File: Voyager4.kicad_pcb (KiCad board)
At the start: 2 copper layers, 34.9 x 38.1 mm, 32 parts, among them Q1 Q_NPN_BEC, SW1 SW_Push, U1 ATmega32U2-MU, U2 PRTR5V0U2X, Y1 16MHz

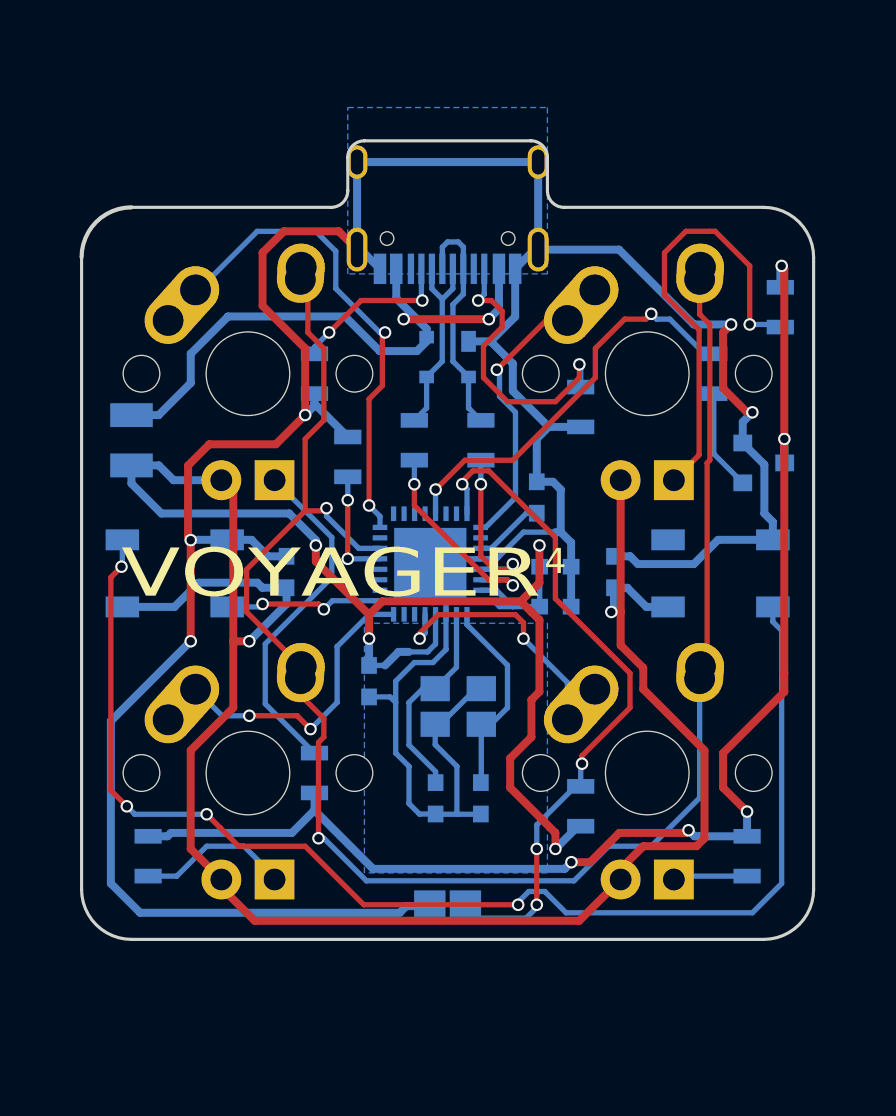
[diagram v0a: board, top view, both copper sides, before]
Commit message: Finish new PCB
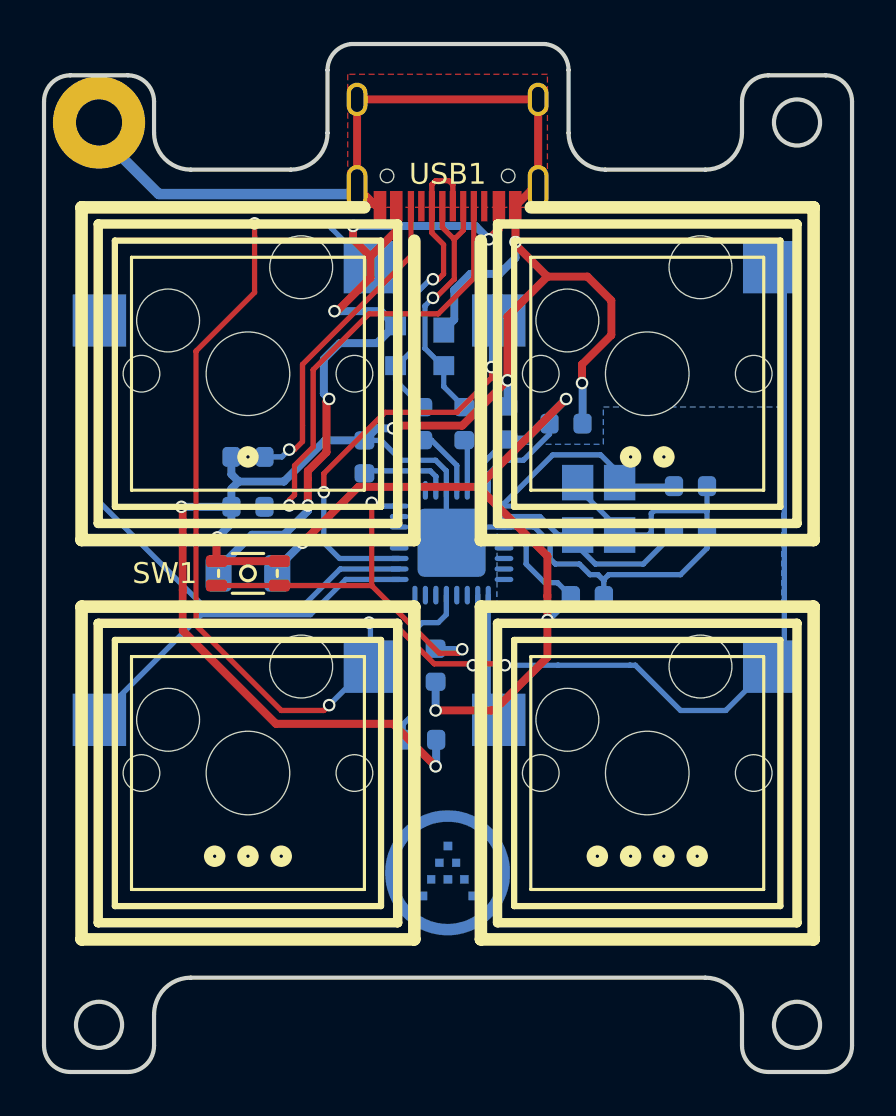
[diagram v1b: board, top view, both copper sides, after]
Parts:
- removed CR1, CR2: 0.1u, Capacitors_SMD:C_0603
- removed D18, D9: WS2812B, LEDs:LED_WS2812B-PLCC4
- removed Q1: Q_NPN_BEC, TO_SOT_Packages_SMD:SOT-23
- removed R10, R27, R7, R8, R9: 1k, Resistors_SMD:R_0805
- added G***: LOGO, locallib:ai-ring-6mm-FancyAss-Mask, B.Cu at (68.3, 63.5)
- added G***: LOGO, locallib:ai-ring-6mm-FancyAss, B.Cu at (68.3, 63.5)
- added GroundingPad: MountingHole_2.2mm_M2_Pad, MountingHole:MountingHole_2.2mm_M2_Pad, F.Cu at (51.6, 27.7)
- added REF**: outline, locallib:outline, F.Cu at (87.8, 25.5)
- C1, C2, C3, C4, C5, C6: footprint Capacitors_SMD:C_0603 -> Capacitor_SMD:C_0603_1608Metric
- F1: footprint Fuse_Holders_and_Fuses:Fuse_SMD1206_Reflow -> Fuse:Fuse_1206_3216Metric
- MX1, MX2, MX3, MX4: footprint MX_Alps_Hybrid:MX-1U -> locallib:MXOnly-1U-Hotswap
- R1, R2, R3, R4, R5, R6: footprint Resistors_SMD:R_0805 -> Resistor_SMD:R_0603_1608Metric
- SW1: footprint random-keyboard-parts:Jumper-UserFriendly-Small -> locallib:Alps-SKSV-LargerPads; moved to F.Cu
- U1: footprint Housings_DFN_QFN:QFN-32-1EP_5x5mm_Pitch0.5mm -> locallib:QFN-32-1EP_5x5mm_Pitch0.5mm
- U2: footprint random-keyboard-parts:SOT143B -> locallib:SOT143B
- USB1: moved to F.Cu
- Y1: footprint Crystals:Crystal_SMD_3225-4pin_3.2x2.5mm -> locallib:Crystal_SMD_3225-4pin_3.2x2.5mm
- moved SW1 18.5 mm to (58.7, 49.2), turned to 0 degrees
- moved C1 17.9 mm to (79.9, 45.1), turned to 0 degrees
- moved C2 17.6 mm to (79.9, 47.2), turned to 0 degrees
- moved R4 16.1 mm to (58.7, 43.7), turned to 180 degrees
- moved C5 14.0 mm to (71.1, 42.0), turned to 90 degrees
- moved R5 13.9 mm to (66.9, 57.1), turned to 180 degrees
- moved Y1 11.6 mm to (75.5, 46.1), turned to 270 degrees
- moved R1 9.65 mm to (67.7, 53.6)
- moved C6 8.75 mm to (73.9, 42.1)
- moved C3 8.45 mm to (64.3, 43.7)
- moved F1 8.44 mm to (58.7, 49.2), turned to 180 degrees
- moved R6 7.10 mm to (58.7, 46.0), turned to 180 degrees
- moved USB1 2.99 mm to (68.3, 24.0), turned to 180 degrees
- moved R3 2.90 mm to (67.1, 42.1)
- moved R2 2.51 mm to (69.1, 42.1)
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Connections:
- U1 pad 10: Net-(U1-Pad10) -> ROW0
- U1 pad 14: ROW0 -> Net-(U1-Pad14)
- U1 pad 16: COL0 -> Net-(U1-Pad16)
- U1 pad 17: Net-(U1-Pad17) -> COL2
- U1 pad 18: Net-(U1-Pad18) -> COL0
- U1 pad 19: Net-(U1-Pad19) -> COL1
- U1 pad 25: COL1 -> Net-(U1-Pad25)
- U1 pad 5: COL3 -> Net-(U1-Pad5)
- U1 pad 8: COL2 -> Net-(U1-Pad8)
- U1 pad 9: RGBLED -> COL3
- U2 pad 2: Net-(R3-Pad1) -> Net-(R2-Pad2)
- U2 pad 3: Net-(R2-Pad2) -> Net-(R3-Pad1)
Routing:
- net +5V: track 143.5 -> 52.9 mm, vias 6 -> 4
- net LEDGND: track 63.1 -> 0.00 mm, vias 5 -> 0
- net Net-(D18-Pad4): track 61.2 -> 0.00 mm, vias 4 -> 0
- net GND: track 175.6 -> 144.2 mm, vias 5 -> 7
- net Net-(MX2-Pad4): track 21.5 -> 0.00 mm, vias 1 -> 0
- net Net-(U1-Pad21): track 19.5 -> 0.00 mm, vias 2 -> 0
- net Net-(MX1-Pad4): track 16.4 -> 0.00 mm
- net Net-(R6-Pad1): track 7.91 -> 21.1 mm, vias 2 -> 1
- net Net-(R1-Pad2): track 32.6 -> 19.7 mm, vias 4 -> 2
- net VCC: track 29.1 -> 37.3 mm, vias 2 -> 5
- net D-: track 10.1 -> 2.46 mm, vias 2 -> 0
- net RGBLED: track 7.62 -> 0.00 mm, vias 2 -> 0
- net Net-(MX3-Pad4): track 7.36 -> 0.00 mm
- net COL1: track 13.1 -> 20.0 mm, vias 1 -> 2
- net COL3: track 12.5 -> 6.15 mm, vias 2 -> 0
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- added copper zone on F.Cu, net GND
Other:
- board size 34.9 x 38.1 mm -> 38.5 x 49 mm
- board text removed: "4"
- board text removed: "R2.0"
- board text removed: "RESET"
- board text removed: "VOYAGER"
- board text removed: "Voyager4"
- board text removed: "kb.ai03.me"
